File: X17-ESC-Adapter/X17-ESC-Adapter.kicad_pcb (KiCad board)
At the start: 2 copper layers, 101.6 x 41.1 mm, 10 parts, among them J2 Power In/Out

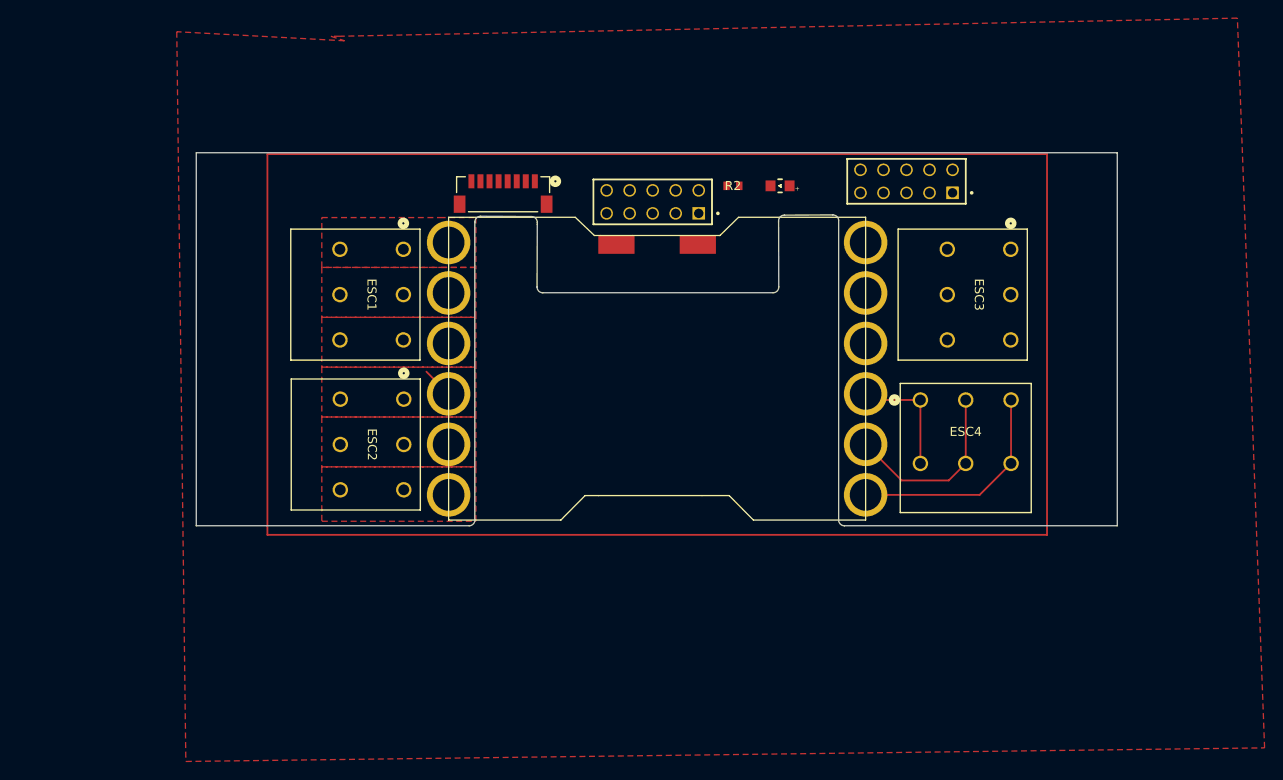
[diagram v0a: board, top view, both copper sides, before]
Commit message: 10/12/24
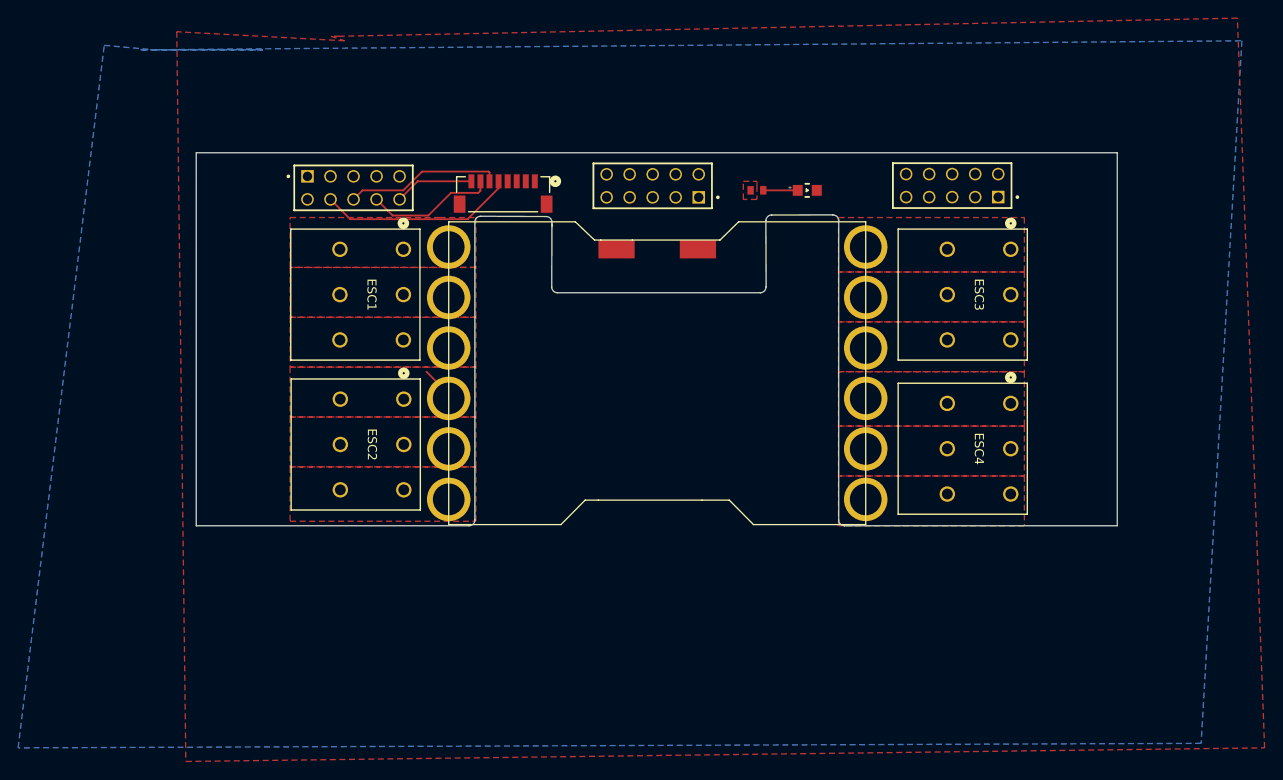
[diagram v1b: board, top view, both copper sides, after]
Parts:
- removed the J2 at (185.5, 80.0)
- moved ESC4 9.97 mm to (197.0, 104.5), turned to -90 degrees
- moved D1 3.04 mm to (174.6, 81.0), turned to 180 degrees
- moved R2 2.70 mm to (169.0, 81.0)
- moved J2 1.77 mm to (157.5, 80.5)
- moved ESC5 0.50 mm to (135.0, 117.9)
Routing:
- net ESC4C: track 24.5 -> 0.00 mm
- net MTR_1: track 0.00 -> 21.6 mm
- net ESC4B: track 20.5 -> 0.00 mm
- net MTR_2: track 0.00 -> 17.3 mm
- net MTR_3: track 0.00 -> 14.4 mm
- net ESC4A: track 13.3 -> 0.95 mm
- net MTR_4: track 0.00 -> 8.75 mm
- net Net-(D1-Pad2): track 0.00 -> 3.80 mm
- added copper zone on B.Cu, net +12V
- added copper zone on F.Cu, net +12V
- added copper zone on F.Cu, net ESC3A
- added copper zone on F.Cu, net ESC3B
- added copper zone on F.Cu, net ESC3C
- added copper zone on F.Cu, net ESC4A
- added copper zone on F.Cu, net ESC4B
- added copper zone on F.Cu, net ESC4C
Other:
- outline, holes or cut-outs redrawn
